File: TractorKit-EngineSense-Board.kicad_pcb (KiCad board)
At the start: 2 copper layers, 57.5 x 45 mm, 24 parts, among them J1 POWER, J2 ADC1, J3 ADC2, J4 UART, J5 I2C, U1 AMS1117-3.3, U2 ACS711xLCTR-12AB, U3 ESP32-WROOM-32

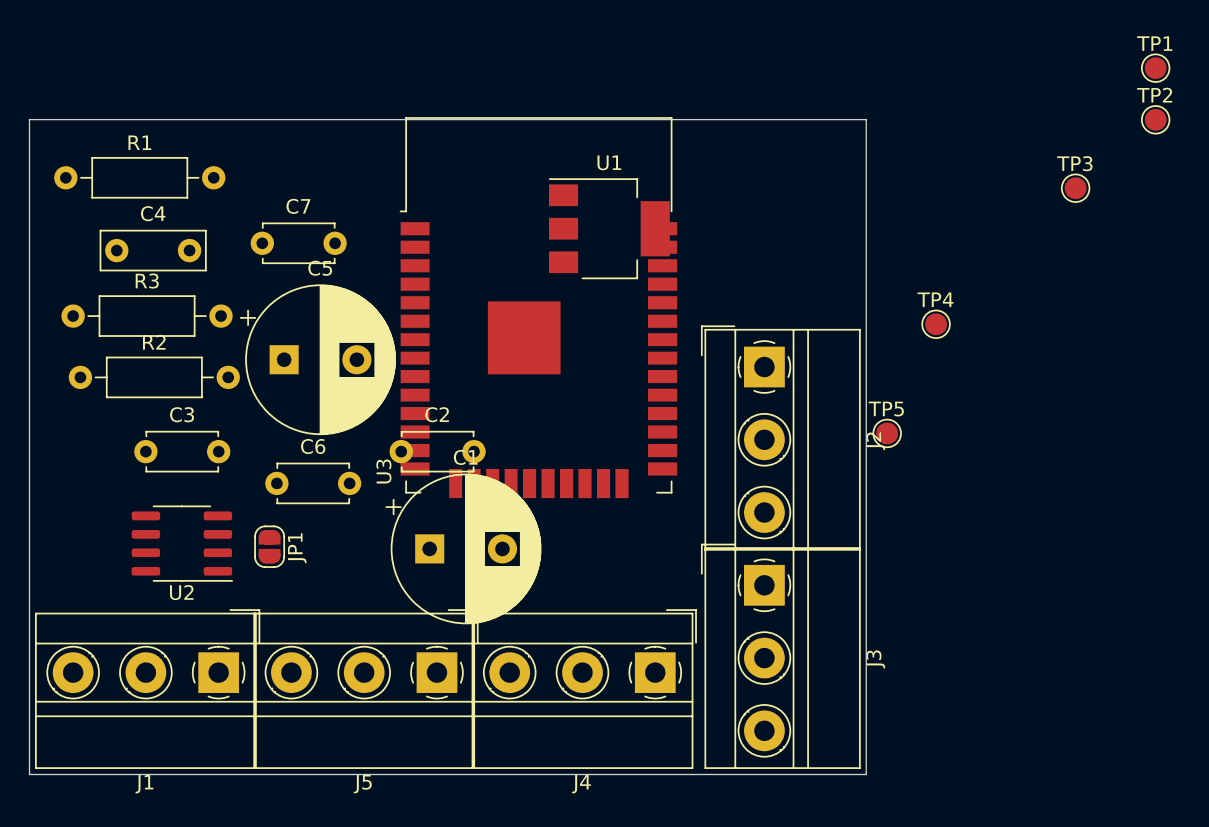
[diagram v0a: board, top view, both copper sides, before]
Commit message: First complete draft.
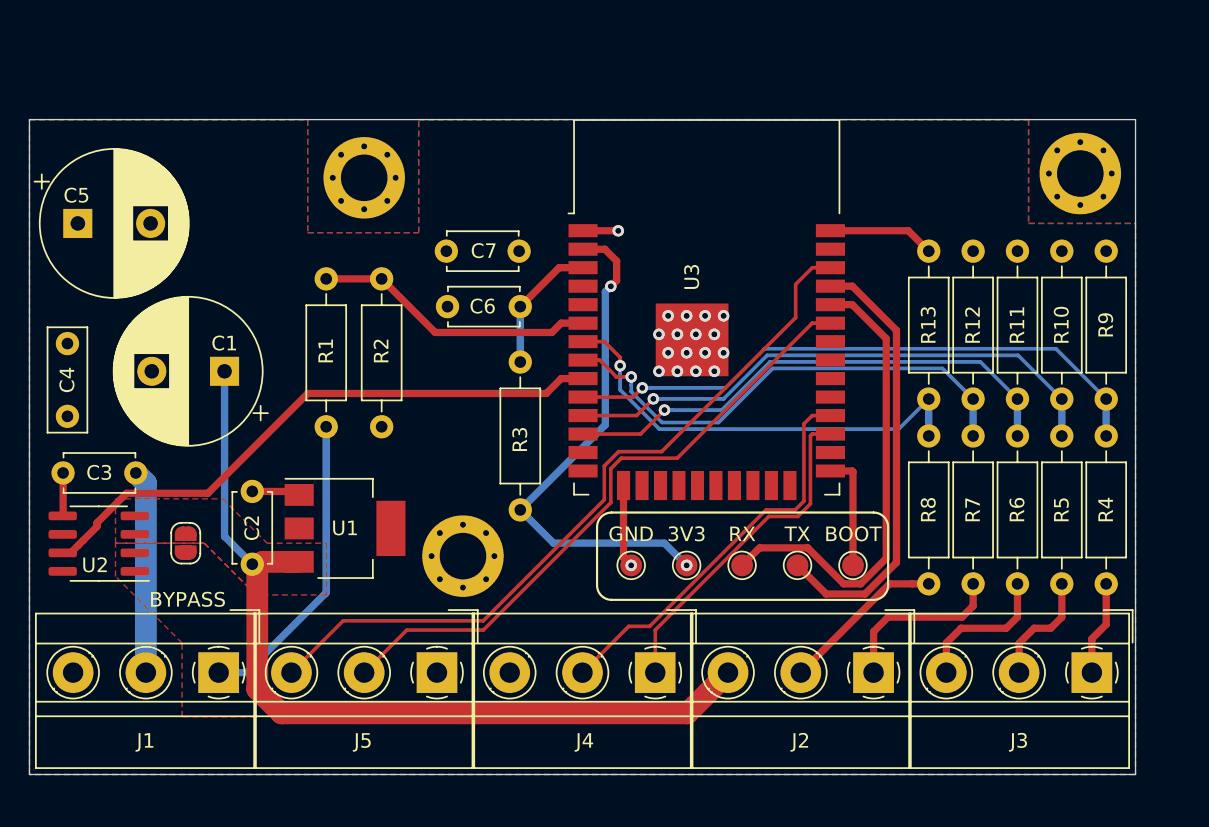
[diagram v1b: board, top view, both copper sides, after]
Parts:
- removed TP1: SERVICE_BOOT, TestPoint:TestPoint_Pad_D1.5mm
- removed TP2: SERVICE_TX, TestPoint:TestPoint_Pad_D1.5mm
- removed TP3: SERVICE_RX, TestPoint:TestPoint_Pad_D1.5mm
- removed TP5: SERVICE_GND, TestPoint:TestPoint_Pad_D1.5mm
- added  : , open-agri.github.io/TKES1, B.Cu at (59.8, 65.2)
- added  : MountingHole_3.2mm_M3_DIN965_Pad, MountingHole:MountingHole_3.2mm_M3_DIN965_Pad, F.Cu at (81.8, 87.0)
- added  : MountingHole_3.2mm_M3_DIN965_Pad, MountingHole:MountingHole_3.2mm_M3_DIN965_Pad, F.Cu at (124.2, 60.7)
- added  : MountingHole_3.2mm_M3_DIN965_Pad, MountingHole:MountingHole_3.2mm_M3_DIN965_Pad, F.Cu at (75.0, 61.0)
- added BOOT: SERVICE_BOOT, TestPoint:TestPoint_Pad_D1.5mm, F.Cu at (108.6, 87.6)
- added GND: SERVICE_GND, TestPoint:TestPoint_Pad_D1.5mm, F.Cu at (93.3, 87.6)
- added R10: 1k, Resistor_THT:R_Axial_DIN0207_L6.3mm_D2.5mm_P10.16mm_Horizontal, F.Cu at (122.9, 76.2)
- added R11: 1k, Resistor_THT:R_Axial_DIN0207_L6.3mm_D2.5mm_P10.16mm_Horizontal, F.Cu at (119.9, 76.2)
- added R12: 1k, Resistor_THT:R_Axial_DIN0207_L6.3mm_D2.5mm_P10.16mm_Horizontal, F.Cu at (116.8, 76.2)
- added R13: 1k, Resistor_THT:R_Axial_DIN0207_L6.3mm_D2.5mm_P10.16mm_Horizontal, F.Cu at (113.8, 76.2)
- added R4: 10k, Resistor_THT:R_Axial_DIN0207_L6.3mm_D2.5mm_P10.16mm_Horizontal, F.Cu at (126.0, 88.9)
- added R5: 10k, Resistor_THT:R_Axial_DIN0207_L6.3mm_D2.5mm_P10.16mm_Horizontal, F.Cu at (122.9, 88.9)
- added R6: 10k, Resistor_THT:R_Axial_DIN0207_L6.3mm_D2.5mm_P10.16mm_Horizontal, F.Cu at (119.9, 88.9)
- added R7: 10k, Resistor_THT:R_Axial_DIN0207_L6.3mm_D2.5mm_P10.16mm_Horizontal, F.Cu at (116.8, 88.9)
- added R8: 10k, Resistor_THT:R_Axial_DIN0207_L6.3mm_D2.5mm_P10.16mm_Horizontal, F.Cu at (113.8, 88.9)
- added R9: 1k, Resistor_THT:R_Axial_DIN0207_L6.3mm_D2.5mm_P10.16mm_Horizontal, F.Cu at (126.0, 76.2)
- added RX: SERVICE_RX, TestPoint:TestPoint_Pad_D1.5mm, F.Cu at (101.0, 87.6)
- added TX: SERVICE_TX, TestPoint:TestPoint_Pad_D1.5mm, F.Cu at (104.8, 87.6)
- moved R3 33.5 mm to (85.7, 83.8), turned to 90 degrees
- moved U1 27.5 mm to (73.7, 85.1)
- moved R1 24.8 mm to (72.4, 78.1), turned to 90 degrees
- moved 3V3 23.8 mm to (97.2, 87.6), turned to 180 degrees
- moved J3 23.3 mm to (125.0, 95.0), turned to 180 degrees
- moved C6 23.1 mm to (85.6, 66.0), turned to 180 degrees
- moved J2 22.3 mm to (110.0, 95.0), turned to 180 degrees
- moved R2 21.8 mm to (76.2, 67.9), turned to 270 degrees
- moved C1 18.6 mm to (65.4, 74.3), turned to 180 degrees
- moved C5 17.0 mm to (55.3, 64.1)
- moved C7 13.4 mm to (80.7, 69.8)
- moved C2 12.8 mm to (67.3, 87.5), turned to 90 degrees
- moved C4 11.9 mm to (54.6, 77.4), turned to 90 degrees
- moved U3 11.5 mm to (98.5, 72.9)
- moved BYPASS 5.77 mm to (62.7, 86.1)
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- renumbered TP4 to 3V3, JP1 to BYPASS
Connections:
- net Net-(J1-Pad1) renamed /12VIN
- J2 pad 1: Net-(J2-Pad1) -> /ADC1_4
- J2 pad 2: Net-(J2-Pad2) -> /ADC1_7
- J2 pad 3: Net-(J2-Pad3) -> +12V
- J3 pad 1: Net-(J3-Pad1) -> /ADC2_8
- J3 pad 2: Net-(J3-Pad2) -> /ADC2_9
- J3 pad 3: Net-(J3-Pad3) -> /ADC2_7
- J4 pad 1: Net-(J4-Pad1) -> /RX
- J4 pad 2: Net-(J4-Pad2) -> /TX
- U3 pad 27: Net-(U3-Pad27) -> /RX
- U3 pad 28: Net-(U3-Pad28) -> /TX
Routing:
- net +12V: track 0.00 -> 59.6 mm
- net /SCL: track 0.00 -> 51.3 mm
- net +3V3: track 0.00 -> 49.5 mm, vias 0 -> 2
- net /SDA: track 0.00 -> 43.3 mm
- net Net-(R4-Pad2): track 0.00 -> 41.3 mm, vias 0 -> 1
- net /AN_CURR: track 0.00 -> 40.9 mm
- net Net-(R10-Pad1): track 0.00 -> 38.4 mm, vias 0 -> 1
- net Net-(R11-Pad1): track 0.00 -> 35.5 mm, vias 0 -> 1
- net Net-(R12-Pad1): track 0.00 -> 34.1 mm, vias 0 -> 1
- net /PR_RX: track 0.00 -> 32.0 mm
- net Net-(R13-Pad1): track 0.00 -> 30.9 mm, vias 0 -> 1
- net /PR_TX: track 0.00 -> 30.3 mm
- net /TX: track 0.00 -> 27.5 mm
- net /RX: track 0.00 -> 23.3 mm
- net GND: track 0.00 -> 21.7 mm, vias 0 -> 18
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- added copper zone on F.Cu, net +12V
- added copper zone on F.Cu, net +3V3
- added copper zone on F.Cu, net /12VIN
- added copper zone on B.Cu, net GND
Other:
- board size 57.5 x 45 mm -> 76 x 45 mm
- rule pad_to_mask_clearance: 0.051 -> 0
- board text added: "+12V"
- board text added: "+3.3V"
- board text added: "0-36V, NOT PROTECTED ALL INPUTS 11k FOR ADC 2 DISABLE Wi-Fi"
- board text added: "12V POWER INPUT 3.3V OUT 1A MAX"
- board text added: "3.3V"
- board text added: "CH4"
- board text added: "CH7"
- board text added: "CH8"
- board text added: "CH9"
- board text added: "EngineSense 1.0 Riccardo Persello ©2020 OpenAgri Model number TKES1 Board S/N: JLCJLCJLCJLC"
- board text added: "GND"
- board text added: "I2C"
- board text added: "INPUT"
- board text added: "IO25"
- board text added: "IO26"
- board text added: "IO27"
- board text added: "OUT"
- board text added: "POWER"
- board text added: "RX"
- board text added: "SAR ADC 1"
- board text added: "SAR ADC 2 / GPIO"
- board text added: "SCL"
- board text added: "SDA"
- board text added: "SERIAL"
- board text added: "SERIAL/I2C 3.3V ONLY NOT PROTECTED NO 5V TOLERANCE"
- board text added: "TX"
